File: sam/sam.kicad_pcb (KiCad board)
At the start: 4 copper layers, 20 x 50 mm, 10 parts, among them J1 USB_A, J2 Conn_Coaxial, U1 SPIRIT1, U2 STM32F070C6Tx, U3 LM3676-3.3

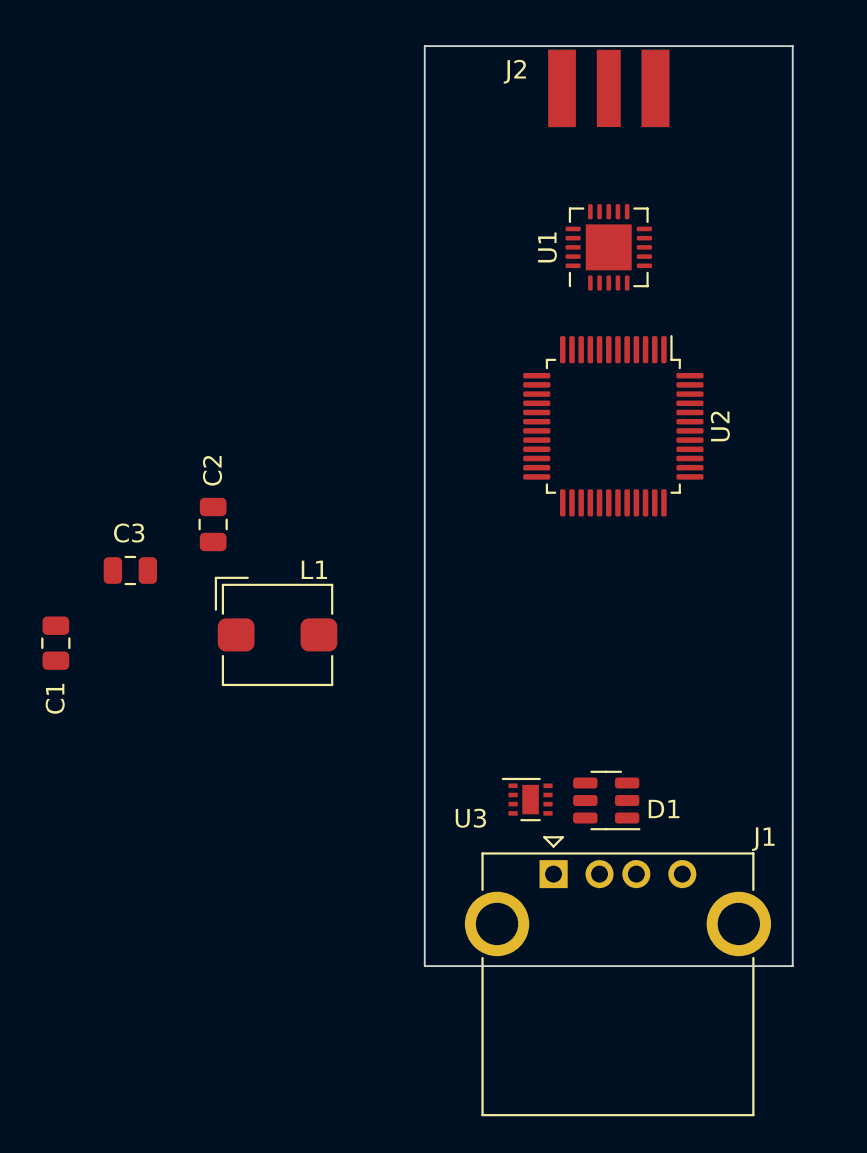
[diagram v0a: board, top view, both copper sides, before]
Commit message: Added low noise LDO and USB plug footprint
A low noise LDO for use in sam has been added, together
with the footprint for a Molex USB A plug.
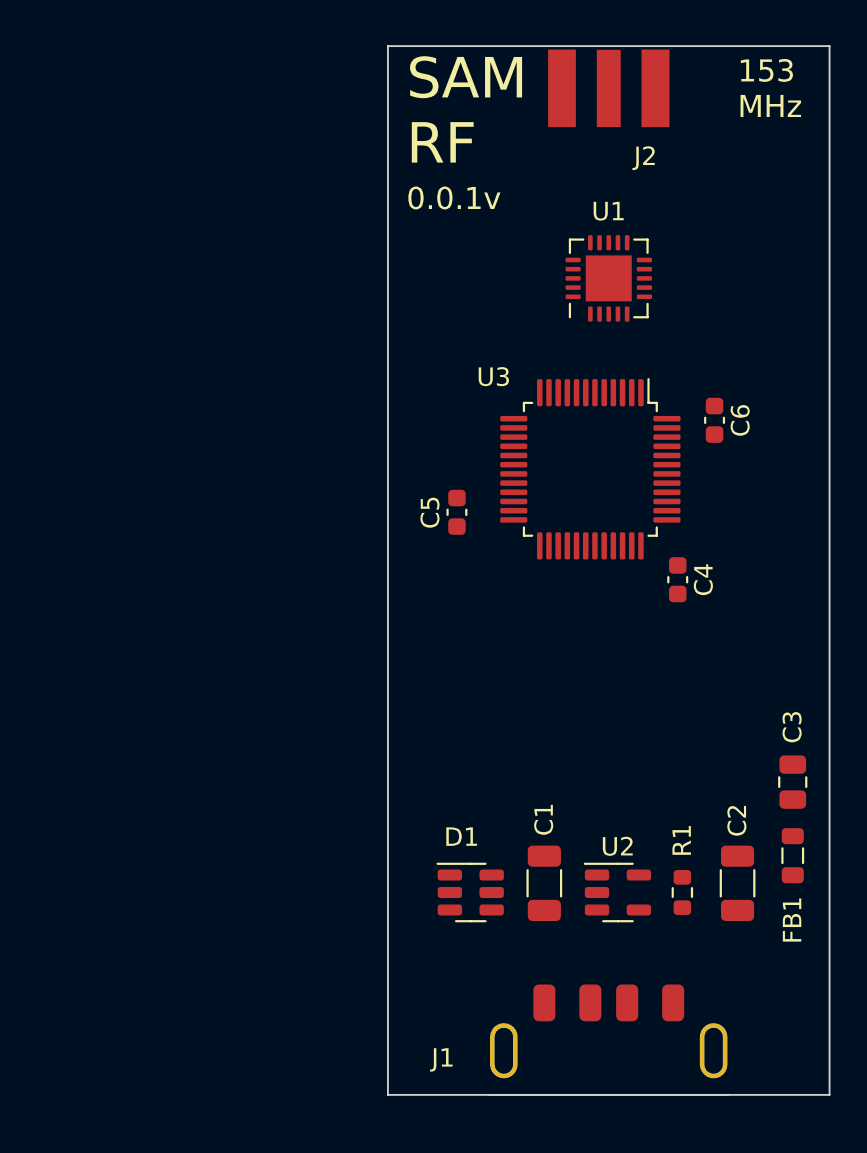
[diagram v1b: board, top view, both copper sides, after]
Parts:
- removed L1: 2u2, Inductor_SMD:L_Bourns_SRP5030T
- removed the U3 at (155.8, 111.0)
- added C4: 100n, Capacitor_SMD:C_0603_1608Metric, F.Cu at (163.8, 99.0)
- added C5: 100n, Capacitor_SMD:C_0603_1608Metric, F.Cu at (151.8, 95.3)
- added C6: 100n, Capacitor_SMD:C_0603_1608Metric, F.Cu at (165.8, 90.3)
- added FB1: FerriteBead, Inductor_SMD:L_0805_2012Metric, F.Cu at (170.0, 114.0)
- added R1: 100k, Resistor_SMD:R_0603_1608Metric, F.Cu at (164.0, 116.0)
- added U2: LDLN030, Package_TO_SOT_SMD:TSOT-23-5, F.Cu at (160.5, 116.0)
- C1: value 4u7 -> 1u; footprint Capacitor_SMD:C_0805_2012Metric -> Capacitor_SMD:C_1206_3216Metric
- C2: value 10u -> 1u; footprint Capacitor_SMD:C_0805_2012Metric -> Capacitor_SMD:C_1206_3216Metric
- J1: footprint Connector_USB:USB_A_CONNFLY_DS1095-WNR0 -> pcrap:USB_A_MOLEX_480372000
- moved C3 37.8 mm to (170.0, 110.0), turned to 90 degrees
- moved C2 34.5 mm to (167.0, 115.5)
- moved C1 29.6 mm to (156.5, 115.5)
- moved J1 9.49 mm to (160.0, 124.0)
- moved D1 8.90 mm to (152.5, 116.0), turned to 0 degrees
- moved U3 2.65 mm to (159.0, 93.0)
- moved U1 1.69 mm to (160.0, 82.6)
- renumbered U2 to U3
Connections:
- C1 pad 1: 5V -> /5V
- C2 pad 1: 3V3 -> /LDO
- D1 pad 4: 5V -> /5V
- D1 pad 6: 5V -> unconnected-(D1-Pad6)
- J1 pad 1: 5V -> /5V
- J1 pad 2: D+ -> D-
- J1 pad 3: D- -> D+
- U3 pad 1: unconnected-(U2-VDD-Pad1) -> 3V3
- U3 pad 23: Net-(U2-VSS-Pad23) -> GND
- U3 pad 24: unconnected-(U2-VDD-Pad24) -> 3V3
- U3 pad 35: Net-(U2-VSS-Pad23) -> GND
- U3 pad 36: unconnected-(U2-VDD-Pad36) -> 3V3
- U3 pad 47: Net-(U2-VSS-Pad23) -> GND
- U3 pad 48: unconnected-(U2-VDD-Pad48) -> 3V3
- U3 pad 8: unconnected-(U2-VSSA-Pad8) -> GND
- U3 pad 9: unconnected-(U2-VDDA-Pad9) -> 3V3
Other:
- board size 20 x 50 mm -> 24 x 57 mm
- board text added: "0.0.1v"
- board text added: "153 MHz"
- board text added: "SAM RF"
